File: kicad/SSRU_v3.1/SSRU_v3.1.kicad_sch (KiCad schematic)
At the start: 89 parts, among them J1 Conn_01x03, J2 Conn_01x24, J3 Conn_02x03_Odd_Even, J31 Conn_01x04, J4 AVR-ISP-6, J5 Conn_01x03, SW1 SW_Push, U1 MCP2515-xSO, U10 TJA1051T, U11 TCA9517D, U12 TJA1051T, U13 CH340N, U2 ATmega328P-A, U4 LM2576S-5, U5 AMS1117-3.3, U7 MCP2515-xSO, U8 74LVC1G17, U9 MT3608/SDB628, Y1 16MHz, Y3 20MHz, Y4 20MHz

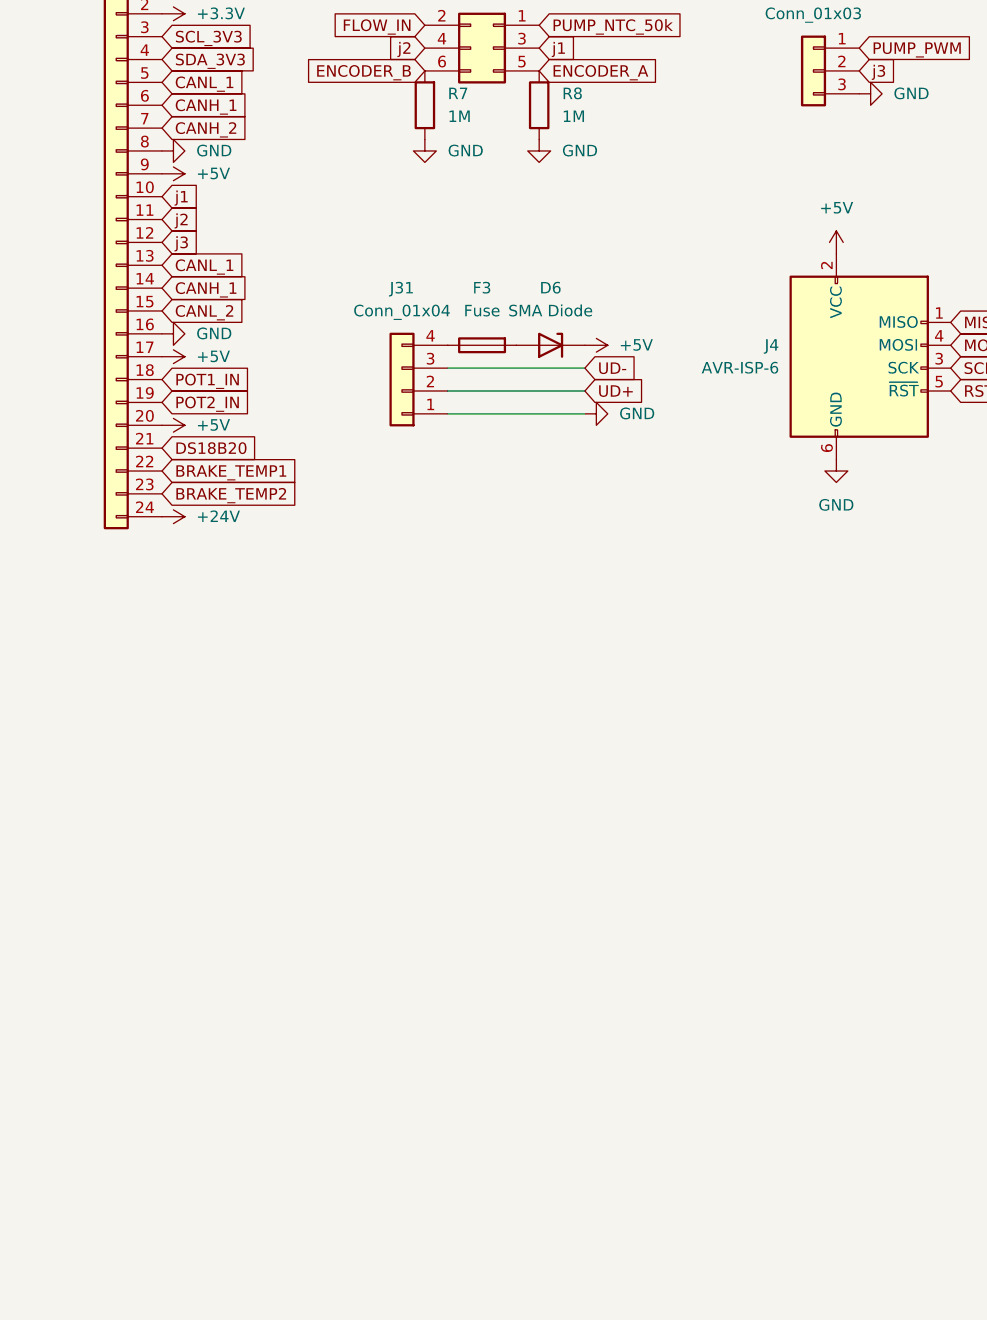
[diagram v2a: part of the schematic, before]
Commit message: ssruv3.1
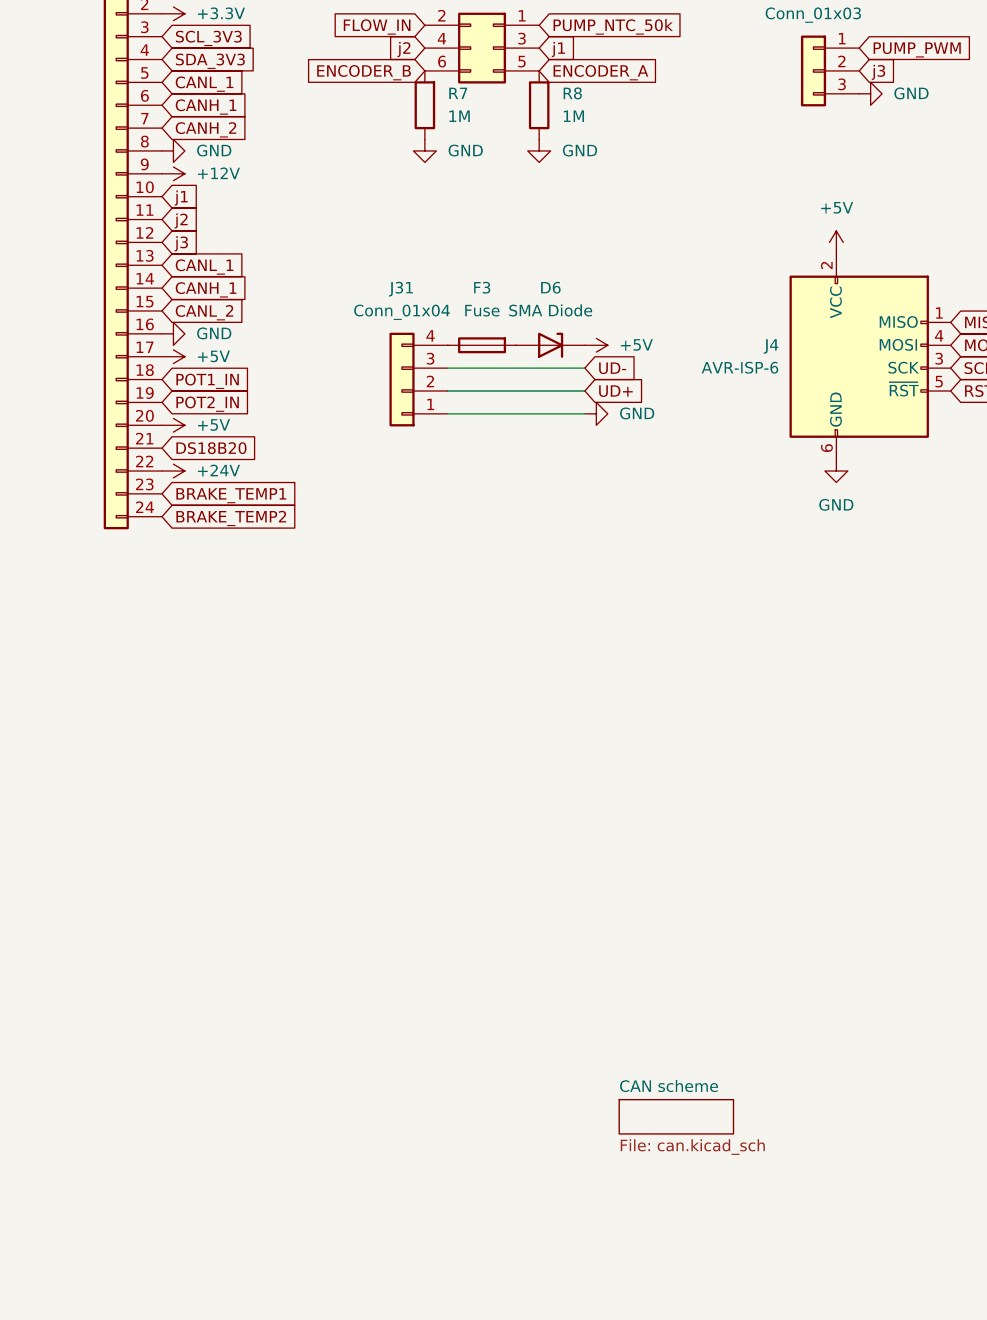
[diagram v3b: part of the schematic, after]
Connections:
- net +12V: now also J2.9 (Pin_9)
- net +24V: now also J2.22 (Pin_22); no longer J2.24 (Pin_24)
- net +5V: no longer J2.9 (Pin_9)
- net BRAKE_TEMP1: now also J2.23 (Pin_23); no longer J2.22 (Pin_22)
- net BRAKE_TEMP2: now also J2.24 (Pin_24); no longer J2.23 (Pin_23)
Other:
- added sheet CAN scheme (can.kicad_sch)
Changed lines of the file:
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@@
 	(global_label "BRAKE_TEMP1"
 		(shape input)
-		(at 303.53 82.55 0)
+		(at 303.53 85.09 0)
 		(fields_autoplaced yes)
 		(effects
@@
 		)
 		(property "Intersheetrefs" "${INTERSHEET_REFS}"
-			(at 319.5779 82.55 0)
+			(at 319.5779 85.09 0)
 			(effects
 				(font
@@
 	(global_label "BRAKE_TEMP2"
 		(shape input)
-		(at 303.53 85.09 0)
+		(at 303.53 87.63 0)
 		(fields_autoplaced yes)
 		(effects
@@
 		)
 		(property "Intersheetrefs" "${INTERSHEET_REFS}"
-			(at 319.5779 85.09 0)
+			(at 319.5779 87.63 0)
 			(effects
 				(font
@@
 	(symbol
 		(lib_id "power:+5V")
-		(at 303.53 49.53 270)
-		(mirror x)
-		(unit 1)
-		(exclude_from_sim no)
-		(in_bom yes)
-		(on_board yes)
-		(dnp no)
-		(fields_autoplaced yes)
-		(property "Reference" "#PWR043"
-			(at 299.72 49.53 0)
-			(effects
-				(font
-					(size 1.27 1.27)
-				)
-				(hide yes)
-			)
-		)
-		(property "Value" "+5V"
-			(at 307.34 49.5299 90)
-			(effects
-				(font
-					(size 1.27 1.27)
-				)
-				(justify left)
-			)
-		)
-		(property "Footprint" ""
-			(at 303.53 49.53 0)
-			(effects
-				(font
-					(size 1.27 1.27)
-				)
-				(hide yes)
-			)
-		)
-		(property "Datasheet" ""
-			(at 303.53 49.53 0)
-			(effects
-				(font
-					(size 1.27 1.27)
-				)
-				(hide yes)
-			)
-		)
-		(property "Description" "Power symbol creates a global label with name \"+5V\""
-			(at 303.53 49.53 0)
-			(effects
-				(font
-					(size 1.27 1.27)
-				)
-				(hide yes)
-			)
-		)
-		(pin "1"
-		)
-		(instances
-			(project "SSRU_v3.1"
-				(path "/bee3e03c-9a5f-4c66-913e-823f7b125a2a"
-					(reference "#PWR043")
-					(unit 1)
-				)
-			)
-		)
-	)
-	(symbol
-		(lib_id "power:+5V")
 		(at 350.52 68.58 270)
 		(mirror x)
@@
 	)
 	(symbol
+		(lib_id "power:+12V")
+		(at 303.53 49.53 270)
+		(mirror x)
+		(unit 1)
+		(exclude_from_sim no)
+		(in_bom yes)
+		(on_board yes)
+		(dnp no)
+		(fields_autoplaced yes)
+		(property "Reference" "#PWR029"
+			(at 299.72 49.53 0)
+			(effects
+				(font
+					(size 1.27 1.27)
+				)
+				(hide yes)
+			)
+		)
+		(property "Value" "+12V"
+			(at 307.34 49.5299 90)
+			(effects
+				(font
+					(size 1.27 1.27)
+				)
+				(justify left)
+			)
+		)
+		(property "Footprint" ""
+			(at 303.53 49.53 0)
+			(effects
+				(font
+					(size 1.27 1.27)
+				)
+				(hide yes)
+			)
+		)
+		(property "Datasheet" ""
+			(at 303.53 49.53 0)
+			(effects
+				(font
+					(size 1.27 1.27)
+				)
+				(hide yes)
+			)
+		)
+		(property "Description" "Power symbol creates a global label with name \"+12V\""
+			(at 303.53 49.53 0)
+			(effects
+				(font
+					(size 1.27 1.27)
+				)
+				(hide yes)
+			)
+		)
+		(pin "1"
+		)
+		(instances
+			(project "SSRU_v3.1"
+				(path "/bee3e03c-9a5f-4c66-913e-823f7b125a2a"
+					(reference "#PWR029")
+					(unit 1)
+				)
+			)
+		)
+	)
+	(symbol
 		(lib_id "Device:C")
 		(at 53.34 22.86 0)
@@
 	(symbol
 		(lib_id "power:+24V")
-		(at 303.53 87.63 270)
+		(at 303.53 82.55 270)
 		(mirror x)
 		(unit 1)
@@
 		(fields_autoplaced yes)
 		(property "Reference" "#PWR061"
-			(at 299.72 87.63 0)
+			(at 299.72 82.55 0)
 			(effects
 				(font
@@
 		)
 		(property "Value" "+24V"
-			(at 307.34 87.6299 90)
+			(at 307.34 82.5499 90)
 			(effects
 				(font
@@
 		)
 		(property "Footprint" ""
-			(at 303.53 87.63 0)
+			(at 303.53 82.55 0)
 			(effects
 				(font
@@
 		)
 		(property "Datasheet" ""
-			(at 303.53 87.63 0)
+			(at 303.53 82.55 0)
 			(effects
 				(font
@@
 		)
 		(property "Description" "Power symbol creates a global label with name \"+24V\""
-			(at 303.53 87.63 0)
+			(at 303.53 82.55 0)
 			(effects
 				(font
@@
 				)
 			)
+		)
+	)
+	(sheet
+		(at 354.33 152.4)
+		(size 12.7 3.81)
+		(exclude_from_sim no)
+		(in_bom yes)
+		(on_board yes)
+		(dnp no)
+		(fields_autoplaced yes)
+		(stroke
+			(width 0.1524)
+			(type solid)
+		)
+		(fill
+			(color 0 0 0 0.0000)
+		)
+		(property "Sheetname" "CAN scheme"
+			(at 354.33 151.6884 0)
+			(effects
+				(font
+					(size 1.27 1.27)
+				)
+				(justify left bottom)
+			)
+		)
+		(property "Sheetfile" "can.kicad_sch"
+			(at 354.33 156.7946 0)
+			(effects
+				(font
+					(size 1.27 1.27)
+				)
+				(justify left top)
+			)
+		)
+		(property "Field2" ""
+			(at 354.33 152.4 0)
+			(effects
+				(font
+					(size 1.27 1.27)
+				)
+			)
+		)
+		(instances
+			(project "SSRU_v3.1"
+				(path "/bee3e03c-9a5f-4c66-913e-823f7b125a2a"
+					(page "3")
+				)
+			)

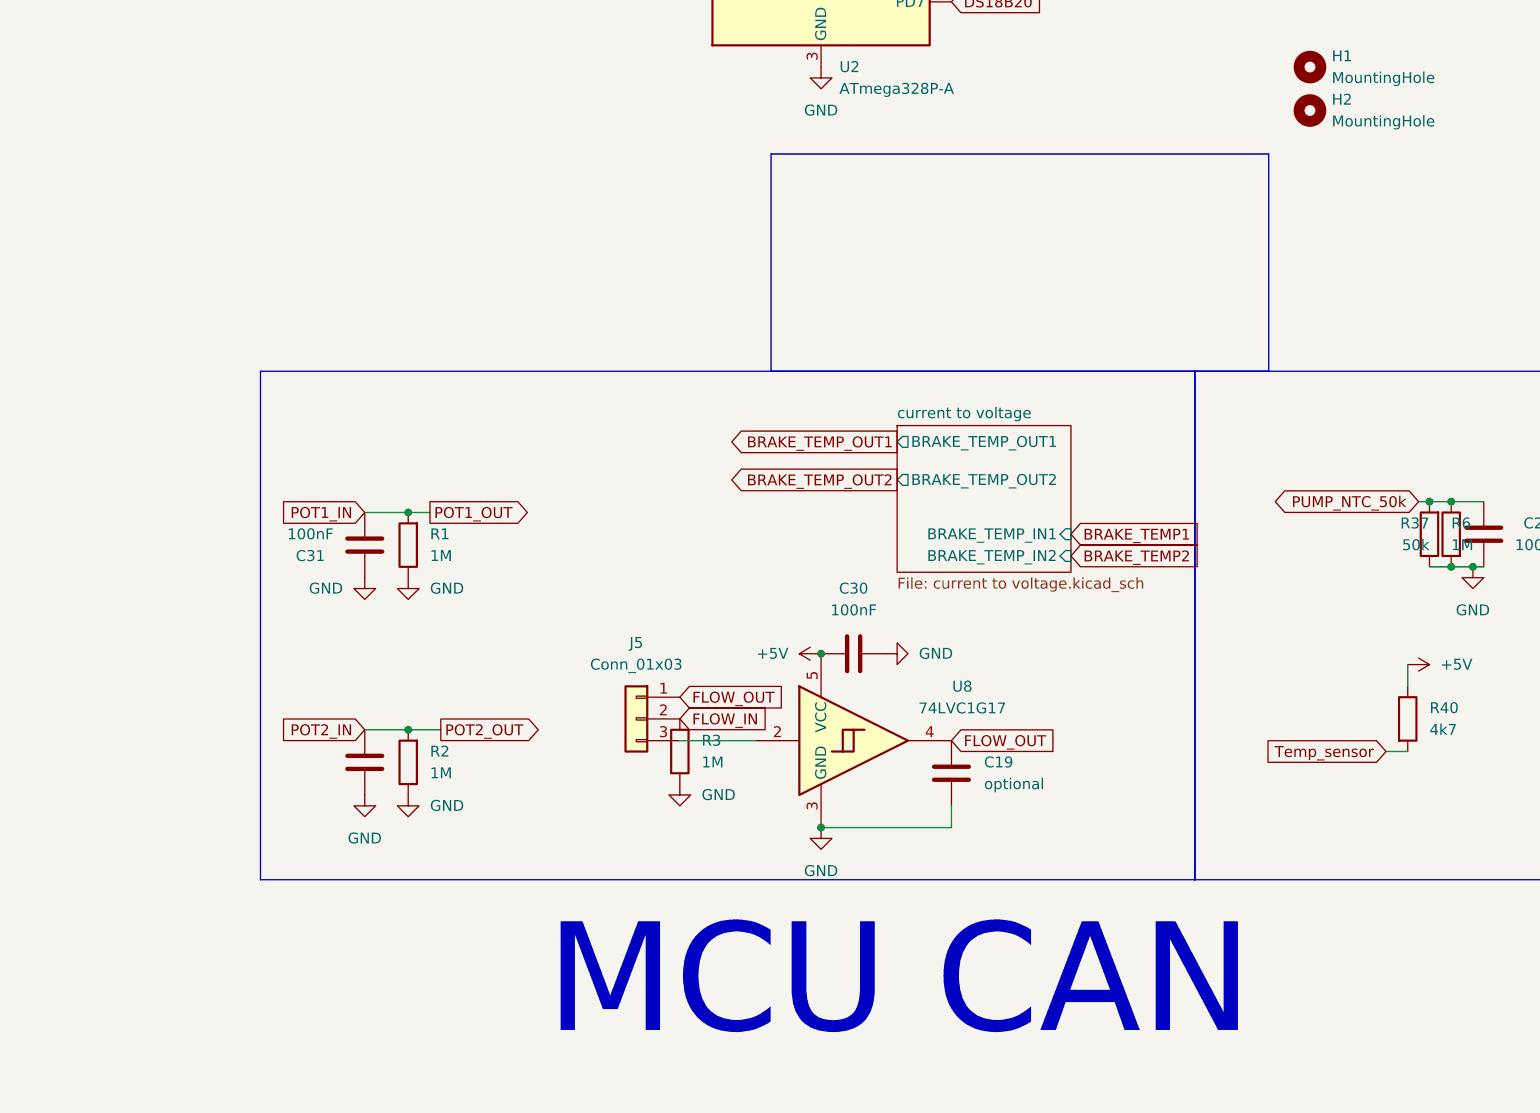
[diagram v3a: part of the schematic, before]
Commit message: ssru
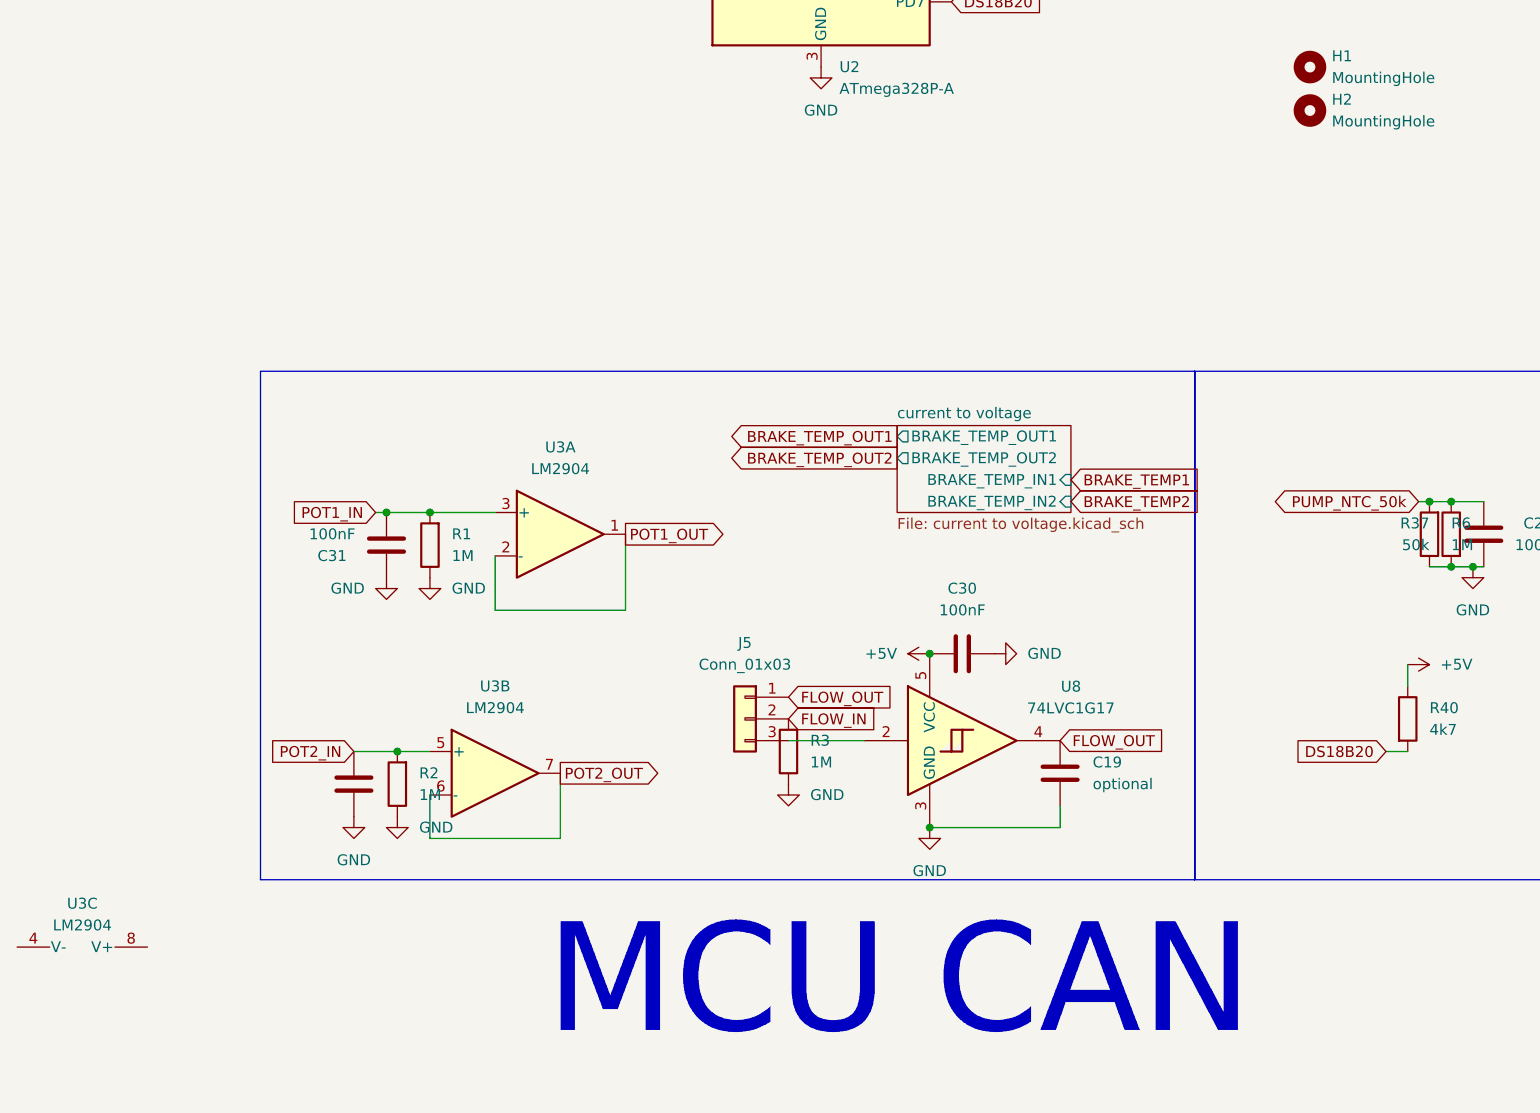
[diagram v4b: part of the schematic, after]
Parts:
- added U3: LM2904, symbol Amplifier_Operational:LM2904
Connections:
- net Temp_sensor is gone; now on net DS18B20: R40.2
- net POT1_IN: now also U3.3 (+); no longer U2.22 (ADC7)
- net POT2_IN: now also U3.5 (+); no longer U2.19 (ADC6)
- new net POT1_OUT: U2.22 (ADC7), U3.1, U3.2 (-)
- new net POT2_OUT: U2.19 (ADC6), U3.6 (-), U3.7
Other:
- moved on the sheet: C19, C30, C31, J5, R1, R2, R3, U8
